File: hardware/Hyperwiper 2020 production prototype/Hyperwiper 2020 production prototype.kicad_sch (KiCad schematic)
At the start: 21 parts, among them K1 Main Power relay, K2 Wiper control relay, Q1 PN2222A, SW1 ON-OFF, U1 Teensy4.0, U3 L7805, X1 W237-3E-bGeigieNanoKit_V1.1r5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, X2 W237-3E-bGeigieNanoKit_V1.1r5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

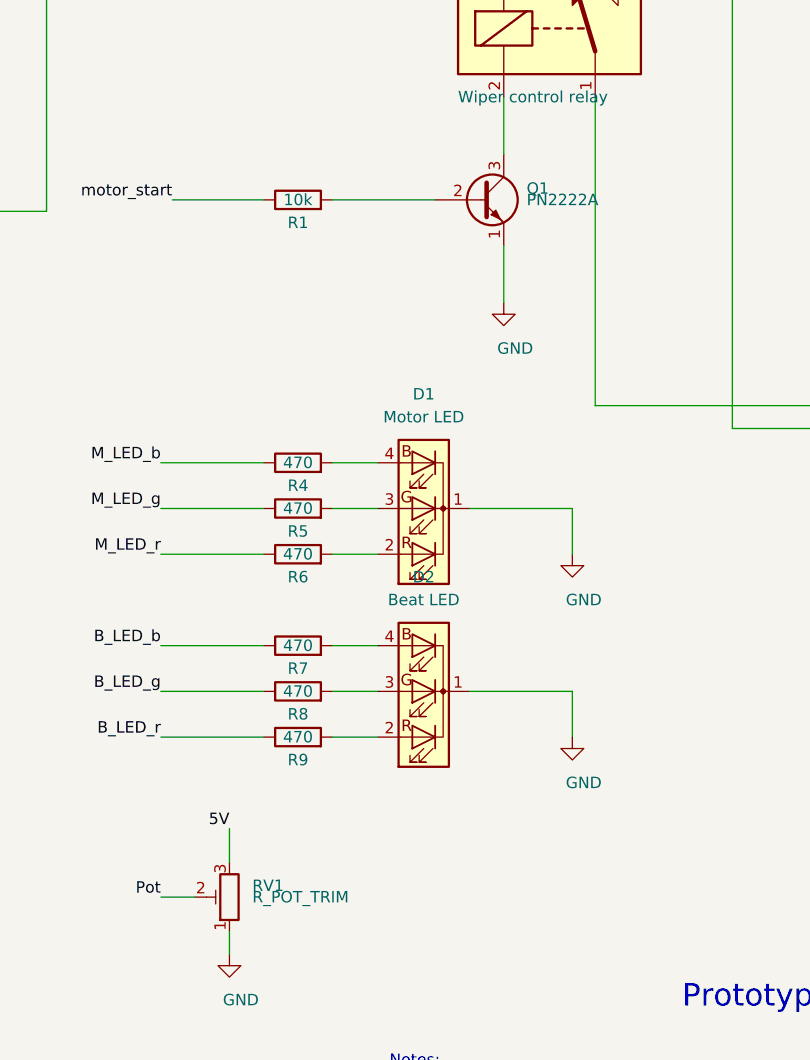
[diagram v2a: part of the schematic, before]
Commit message: Updated board
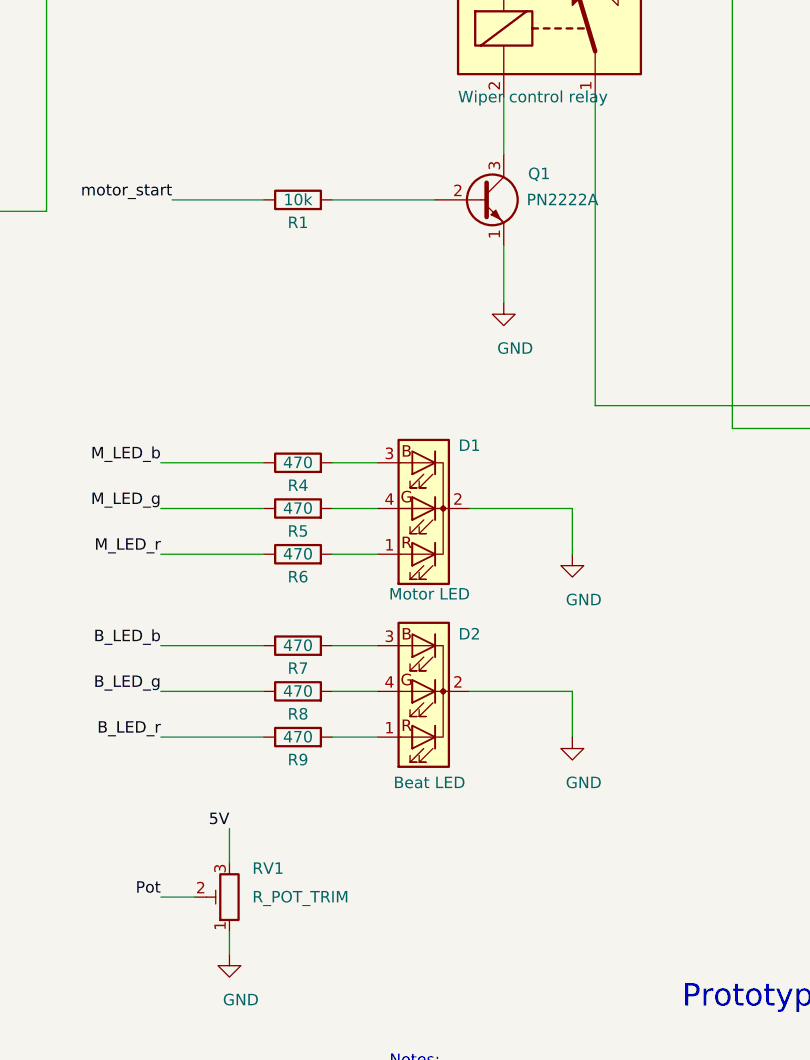
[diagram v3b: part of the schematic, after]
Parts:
- removed D1: Motor LED, LED_THT:LED_D5.0mm-4_RGB, symbol Device:LED_CRGB
- removed D2: Beat LED, LED_THT:LED_D5.0mm-4_RGB, symbol Device:LED_CRGB
- added D1: Motor LED, LED_THT:LED_D5.0mm-4_RGB, symbol Device:LED_RCBG
- added D2: Beat LED, LED_THT:LED_D5.0mm-4_RGB, symbol Device:LED_RCBG
- SW1: footprint (none) -> Button_Switch_THT:SW_Tactile_SPST_Angled_PTS645Vx83-2LFS
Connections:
- net GND: now also D1.2 (K), D2.2 (K)
- net at R6.2: now also D1.1 (RA)
- net at R5.2: now also D1.4 (GA)
- net at R4.2: now also D1.3 (BA)
- net at R7.2: now also D2.3 (BA)
- net at R8.2: now also D2.4 (GA)
- net at R9.2: now also D2.1 (RA)
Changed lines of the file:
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@@
-(kicad_sch (version 20200714) (host eeschema "5.99.0-unknown-27d319b2d~89~ubuntu20.04.1")
+(kicad_sch (version 20200714) (host eeschema "5.99.0-unknown-8c94d88c7~89~ubuntu20.04.1")
   (page 1 1)
   (paper "A4")
@@
     (property "Reference" "SW1" (id 0) (at 238.76 88.9 0))
     (property "Value" "ON-OFF" (id 1) (at 250.19 88.9 90))
-    (property "Footprint" "" (id 2) (at 245.11 88.9 0)
+    (property "Footprint" "Button_Switch_THT:SW_Tactile_SPST_Angled_PTS645Vx83-2LFS" (id 2) (at 245.11 88.9 0)
       (effects (font (size 1.27 1.27)) hide)
     )
@@
   (symbol (lib_id "Device:R_POT_TRIM") (at 161.29 160.02 180) (unit 1)
     (in_bom yes) (on_board yes)
-    (property "Reference" "RV1" (id 0) (at 163.83 158.75 0)
+    (property "Reference" "RV1" (id 0) (at 163.83 156.845 0)
       (effects (font (size 1.27 1.27)) (justify right))
     )
@@
   (symbol (lib_id "Transistor_BJT:PN2222A") (at 189.23 82.55 0) (unit 1)
     (in_bom yes) (on_board yes)
-    (property "Reference" "Q1" (id 0) (at 194.31 81.28 0)
+    (property "Reference" "Q1" (id 0) (at 194.4624 79.6544 0)
       (effects (font (size 1.27 1.27)) (justify left))
     )
@@
     )
   )
-  (symbol (lib_id "Device:LED_CRGB") (at 182.88 116.84 180) (unit 1)
-    (in_bom yes) (on_board yes)
-    (property "Reference" "D1" (id 0) (at 182.88 104.14 0))
-    (property "Value" "Motor LED" (id 1) (at 182.88 106.68 0))
+  (symbol (lib_id "Device:LED_RCBG") (at 182.88 116.84 180) (unit 1)
+    (in_bom yes) (on_board yes)
+    (property "Reference" "D1" (id 0) (at 187.96 109.855 0))
+    (property "Value" "Motor LED" (id 1) (at 183.515 126.365 0))
     (property "Footprint" "LED_THT:LED_D5.0mm-4_RGB" (id 2) (at 182.88 115.57 0)
       (effects (font (size 1.27 1.27)) hide)
@@
     )
   )
-  (symbol (lib_id "Device:LED_CRGB") (at 182.88 137.16 180) (unit 1)
-    (in_bom yes) (on_board yes)
-    (property "Reference" "D2" (id 0) (at 182.88 124.46 0))
-    (property "Value" "Beat LED" (id 1) (at 182.88 127 0))
+  (symbol (lib_id "Device:LED_RCBG") (at 182.88 137.16 180) (unit 1)
+    (in_bom yes) (on_board yes)
+    (property "Reference" "D2" (id 0) (at 187.96 130.81 0))
+    (property "Value" "Beat LED" (id 1) (at 183.515 147.32 0))
     (property "Footprint" "LED_THT:LED_D5.0mm-4_RGB" (id 2) (at 182.88 135.89 0)
       (effects (font (size 1.27 1.27)) hide)
@@
       (reference "#PWR0110") (unit 1)
     )
-    (path "/3e7c7f71-990b-4b23-8faa-21bc92ed5e62"
+    (path "/2723ac12-21fb-4eb0-b91d-4ea3a28c8ae0"
       (reference "D1") (unit 1)
     )
-    (path "/83ccb75b-41e2-4da1-b59a-2bb55bc93cc7"
+    (path "/a626228a-9c73-4fcc-9148-d4b02f6a1a48"
       (reference "D2") (unit 1)
     )
